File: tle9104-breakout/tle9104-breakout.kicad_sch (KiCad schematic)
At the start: 20 parts, among them J1 Conn_01x13, J2 Conn_01x03_Female, J3 Conn_01x03_Female, J4 Conn_01x13, J5 Conn_01x03_Female, U1 TLE9104SH

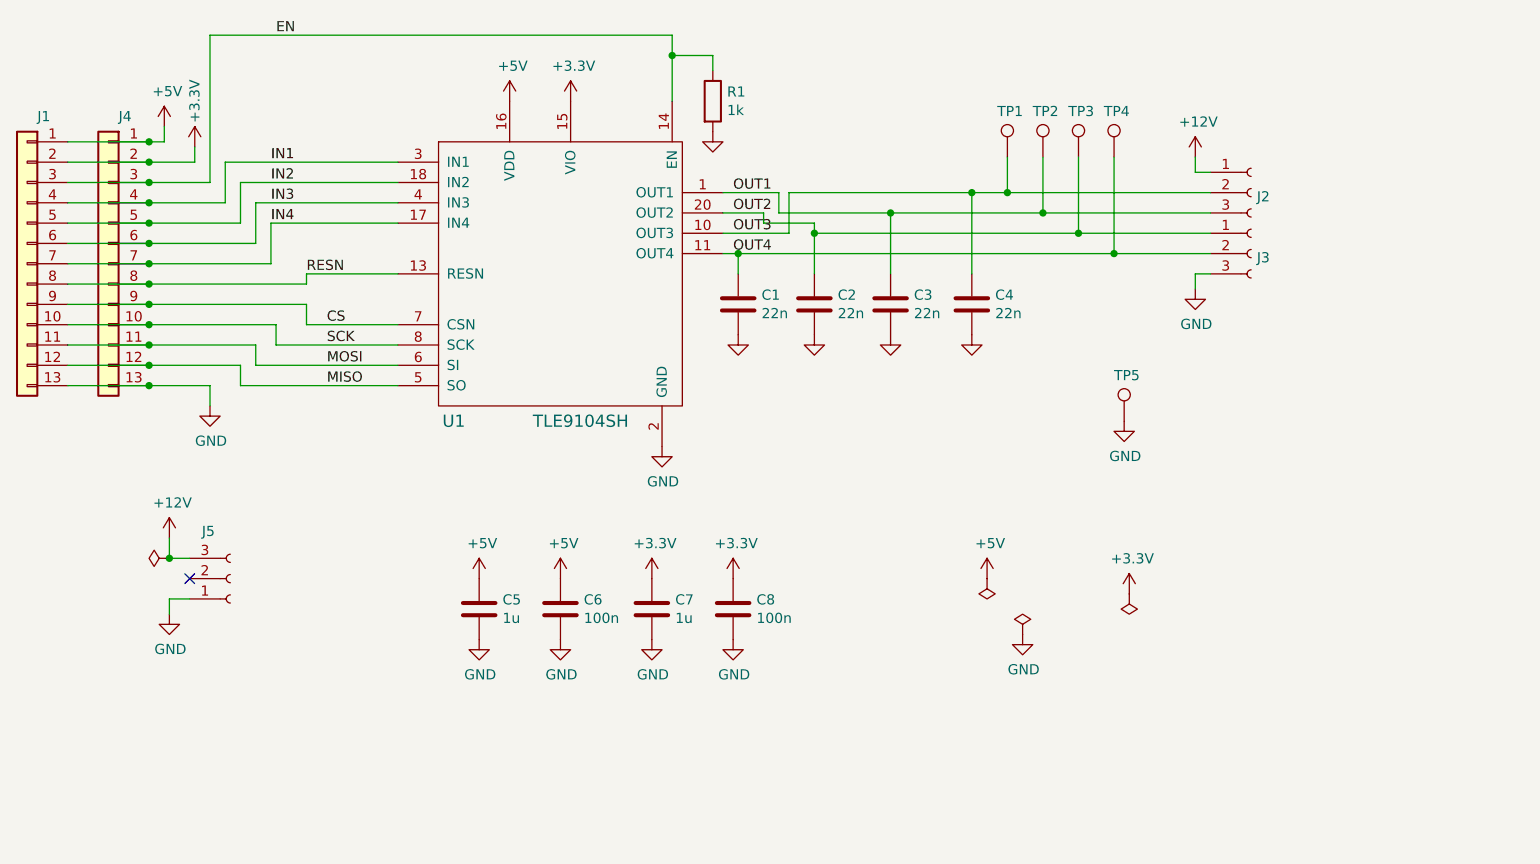
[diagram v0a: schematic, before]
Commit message: #261
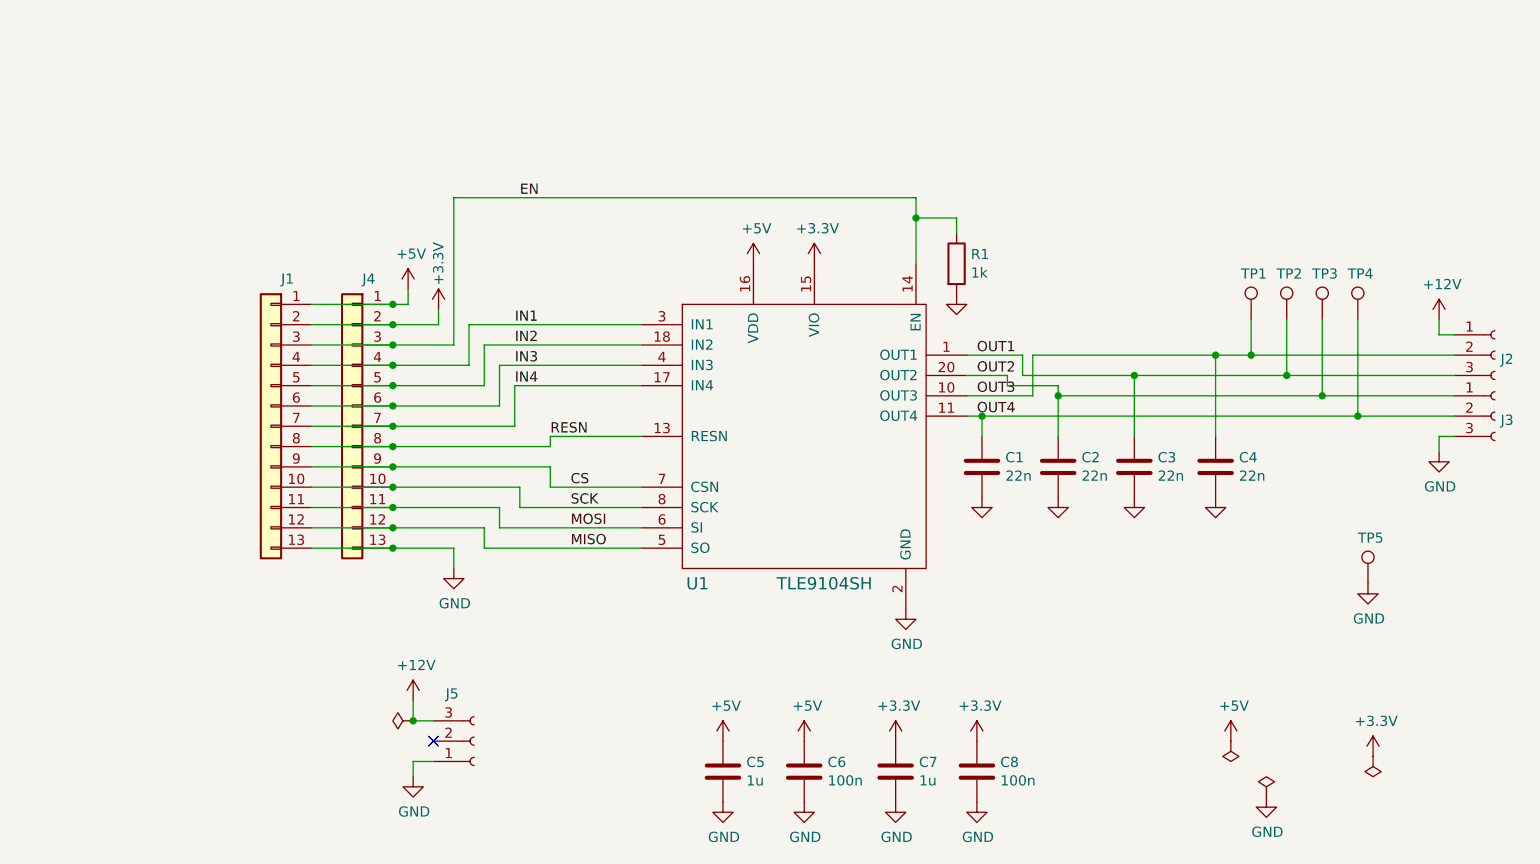
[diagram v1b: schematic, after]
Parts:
- C1, C2, C3, C4: LCSC (none) -> C21122
- C5, C7: LCSC (none) -> C15849
- C6, C8: LCSC (none) -> C307331
- R1: LCSC (none) -> C21190
- U1: LCSC (none) -> C2650386
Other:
- moved on the sheet: C1, C5, C6, J1, J2, J3, J4, J5, R1, TP1, TP2, TP3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
